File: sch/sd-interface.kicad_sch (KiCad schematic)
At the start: 34 parts, among them J5 F32Q-1A7H1-11022, J6 5V_out, J7 MEM2075-00-140-01-A, Q1 Q_PMOS_GSD, U3 CD4043BDR, U4 MAX4996LETG_, U5 TPS22919DCKR

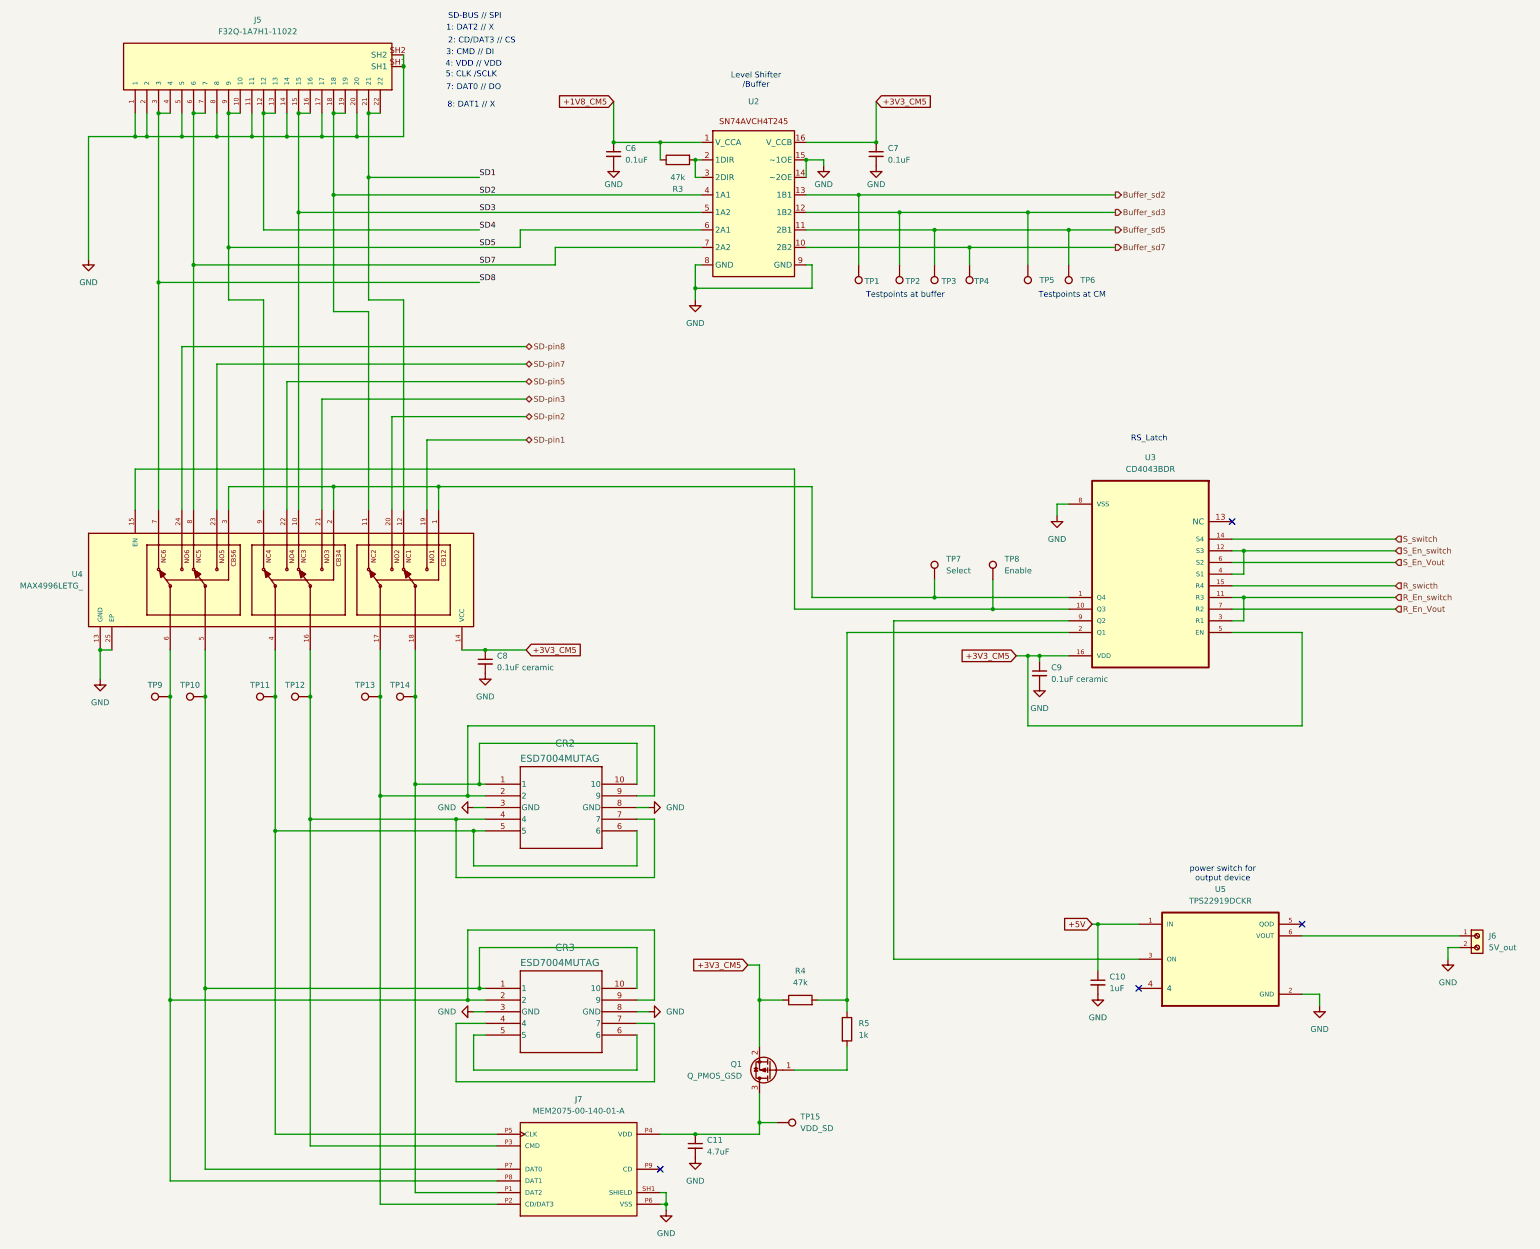
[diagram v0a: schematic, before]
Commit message: Fjernet gammelt og la til nye komponenter, merging ferdig
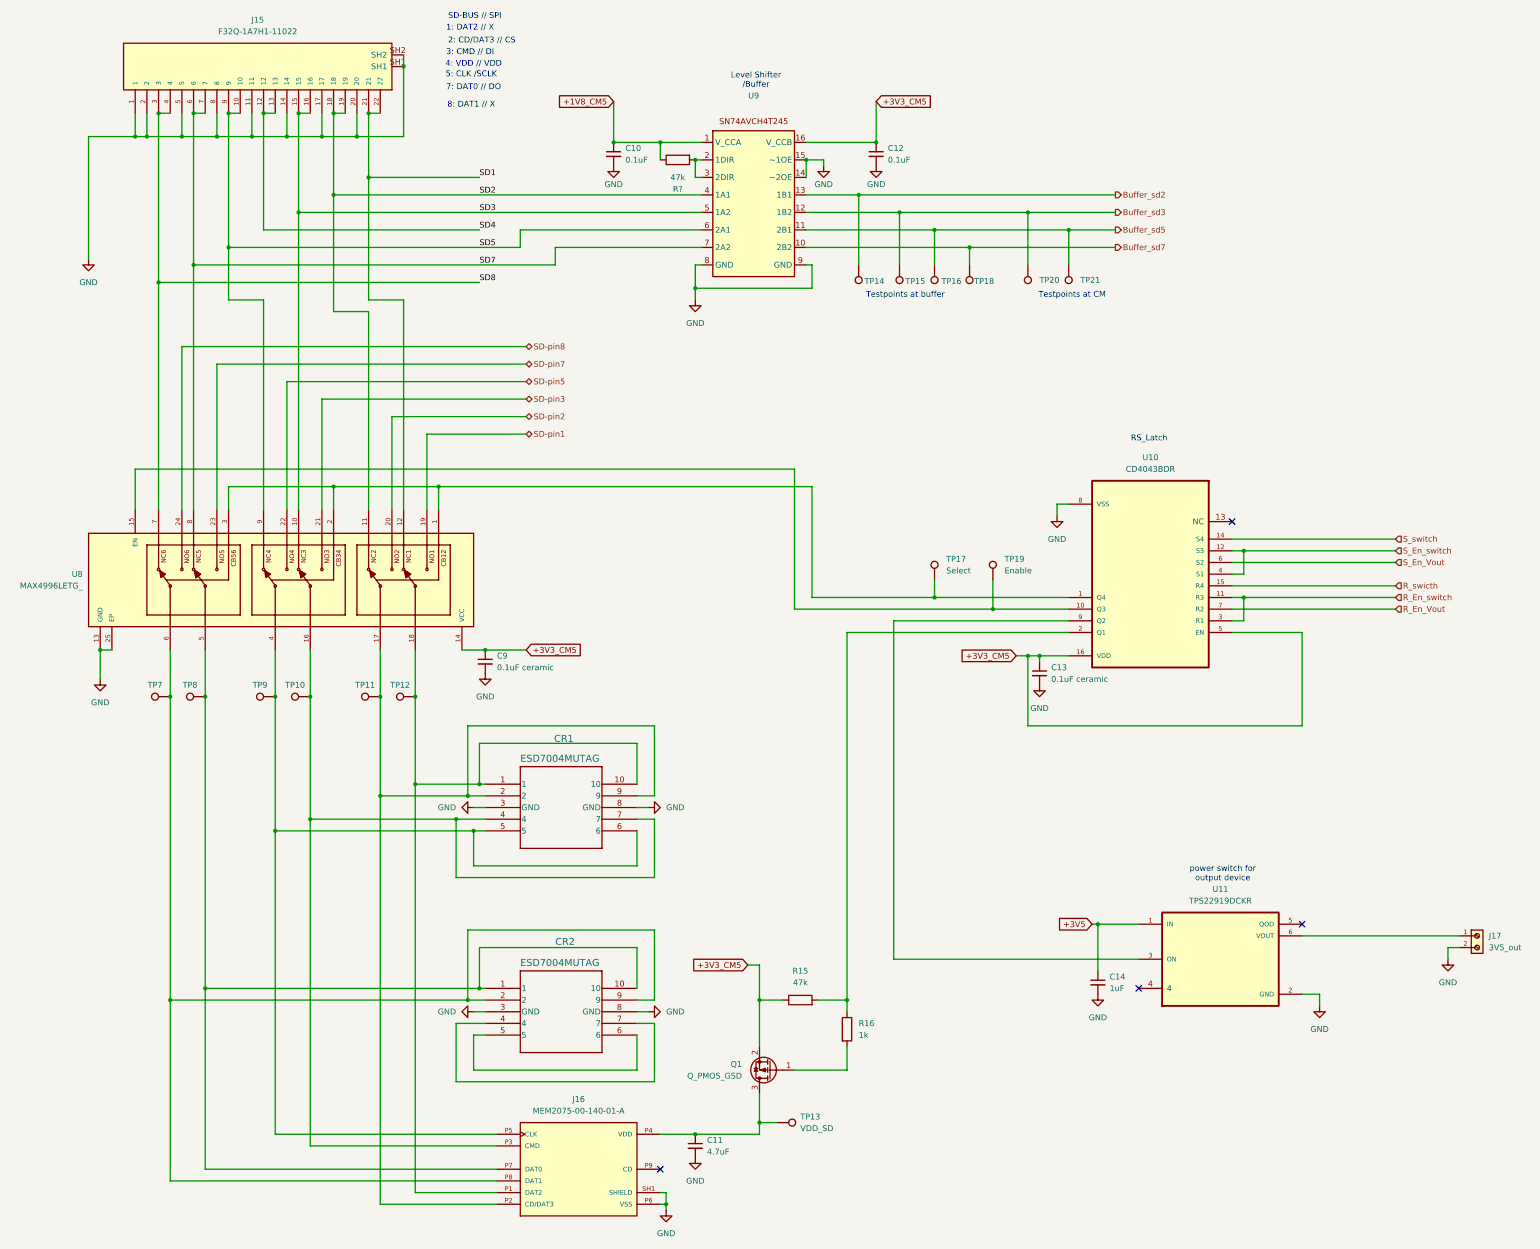
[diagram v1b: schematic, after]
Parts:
- J17: renamed from J6; value 5V_out -> 3V5_out
- renumbered C6 to C10, C7 to C12, C9 to C13, C10 to C14, C8 to C9, CR2 to CR1, CR3 to CR2, J5 to J15, J7 to J16, R4 to R15, R5 to R16, R3 to R?, TP12 to TP10, TP13 to TP11, TP14 to TP12, TP15 to TP13, TP1 to TP14, TP2 to TP15, TP3 to TP16, TP7 to TP17, TP4 to TP18, TP8 to TP19, TP5 to TP20, TP6 to TP21, TP9 to TP7, TP10 to TP8, TP11 to TP9, U3 to U10, U5 to U11, U4 to U8, U2 to U9
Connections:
- net +5V renamed +3V5
